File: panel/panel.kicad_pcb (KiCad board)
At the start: 2 copper layers, 70.9 x 128.5 mm, 0 parts

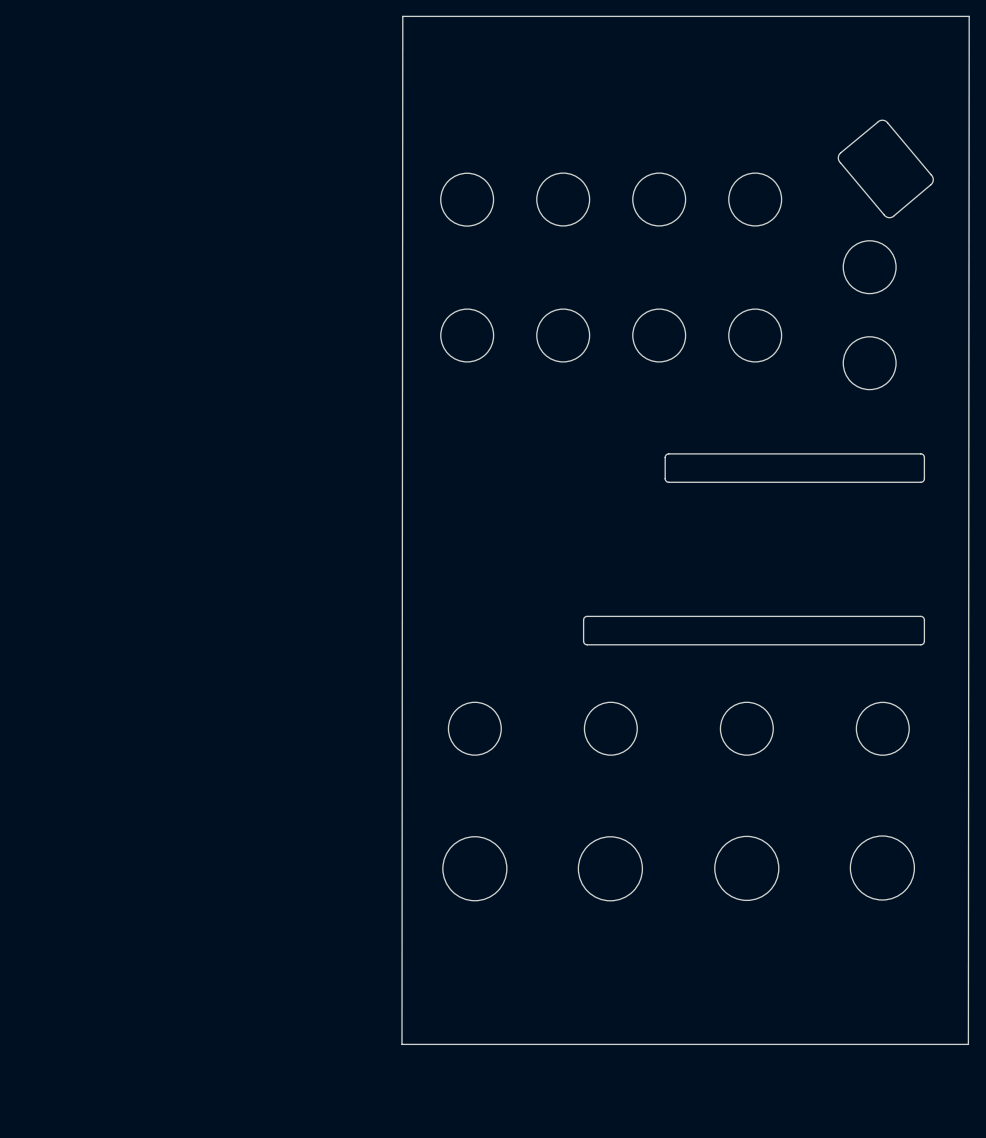
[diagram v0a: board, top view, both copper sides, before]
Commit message: Panel artwork done
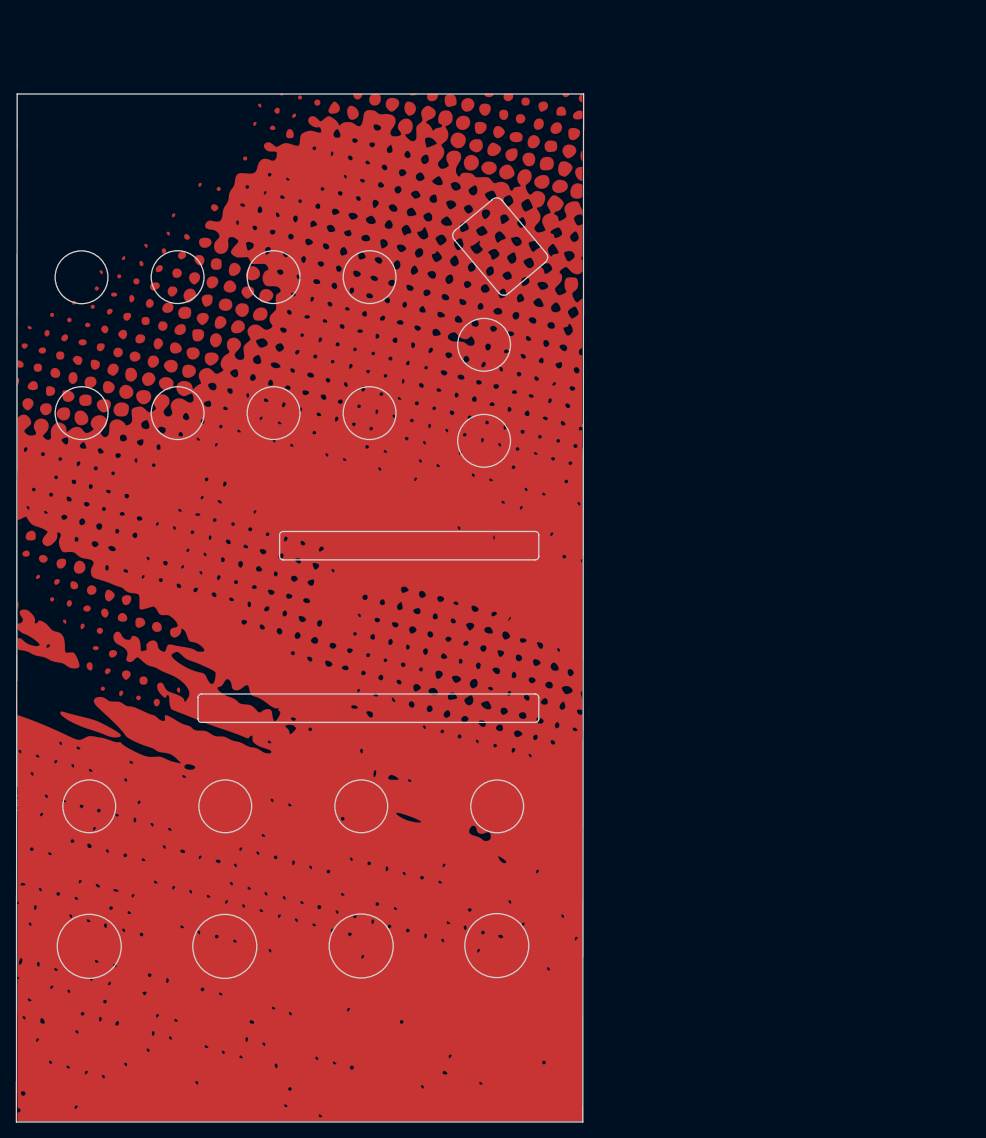
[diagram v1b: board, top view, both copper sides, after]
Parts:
- added G*** (x2): LOGO, LOGO, F.Cu at (104.8, 98.5)
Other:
- outline, holes or cut-outs redrawn
- net class Default: via_dia 0.8 -> 0.6
- rule pad_to_mask_clearance: 0.05 -> 0.2
